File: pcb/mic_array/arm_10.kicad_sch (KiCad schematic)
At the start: 16 parts, among them U81 IM72D128V01XTMA1, U82 IM72D128V01XTMA1, U83 IM72D128V01XTMA1, U84 IM72D128V01XTMA1, U85 IM72D128V01XTMA1, U86 IM72D128V01XTMA1, U87 IM72D128V01XTMA1, U88 IM72D128V01XTMA1

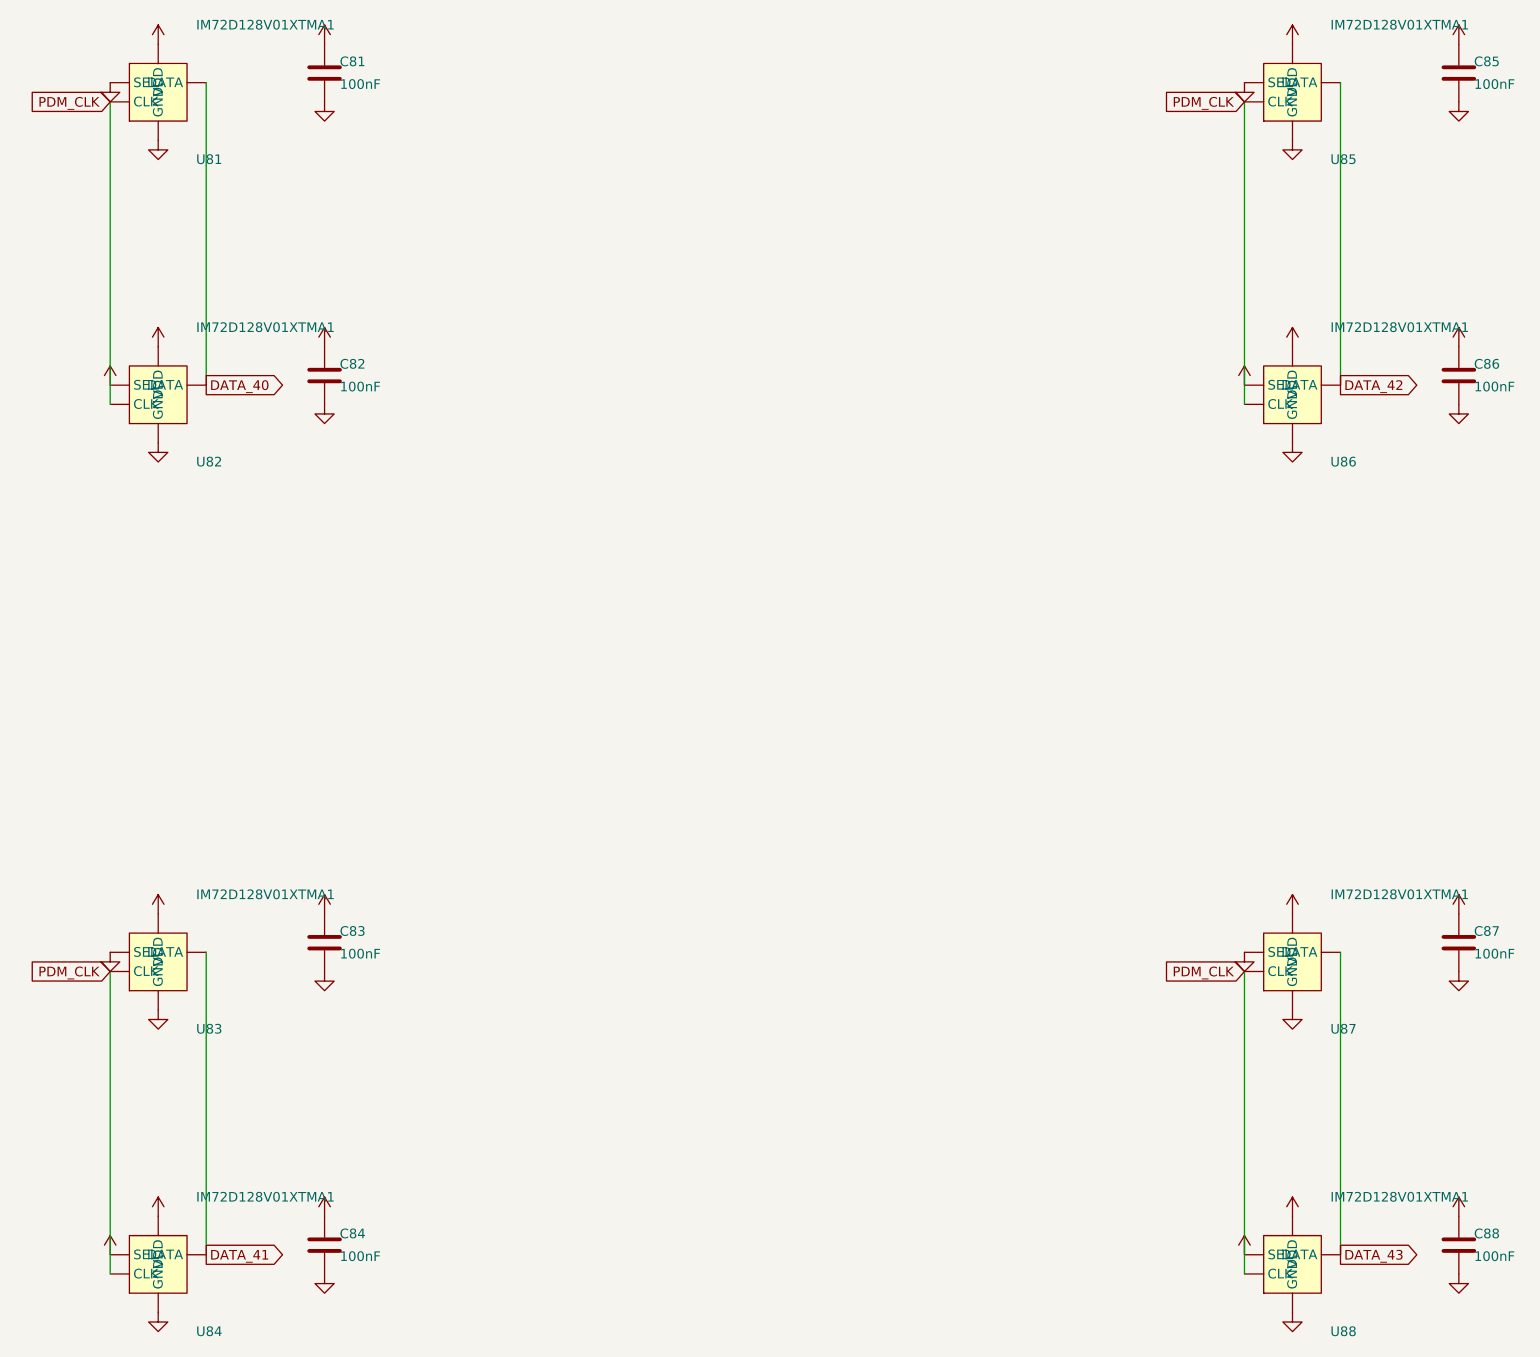
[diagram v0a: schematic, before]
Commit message: Updated.
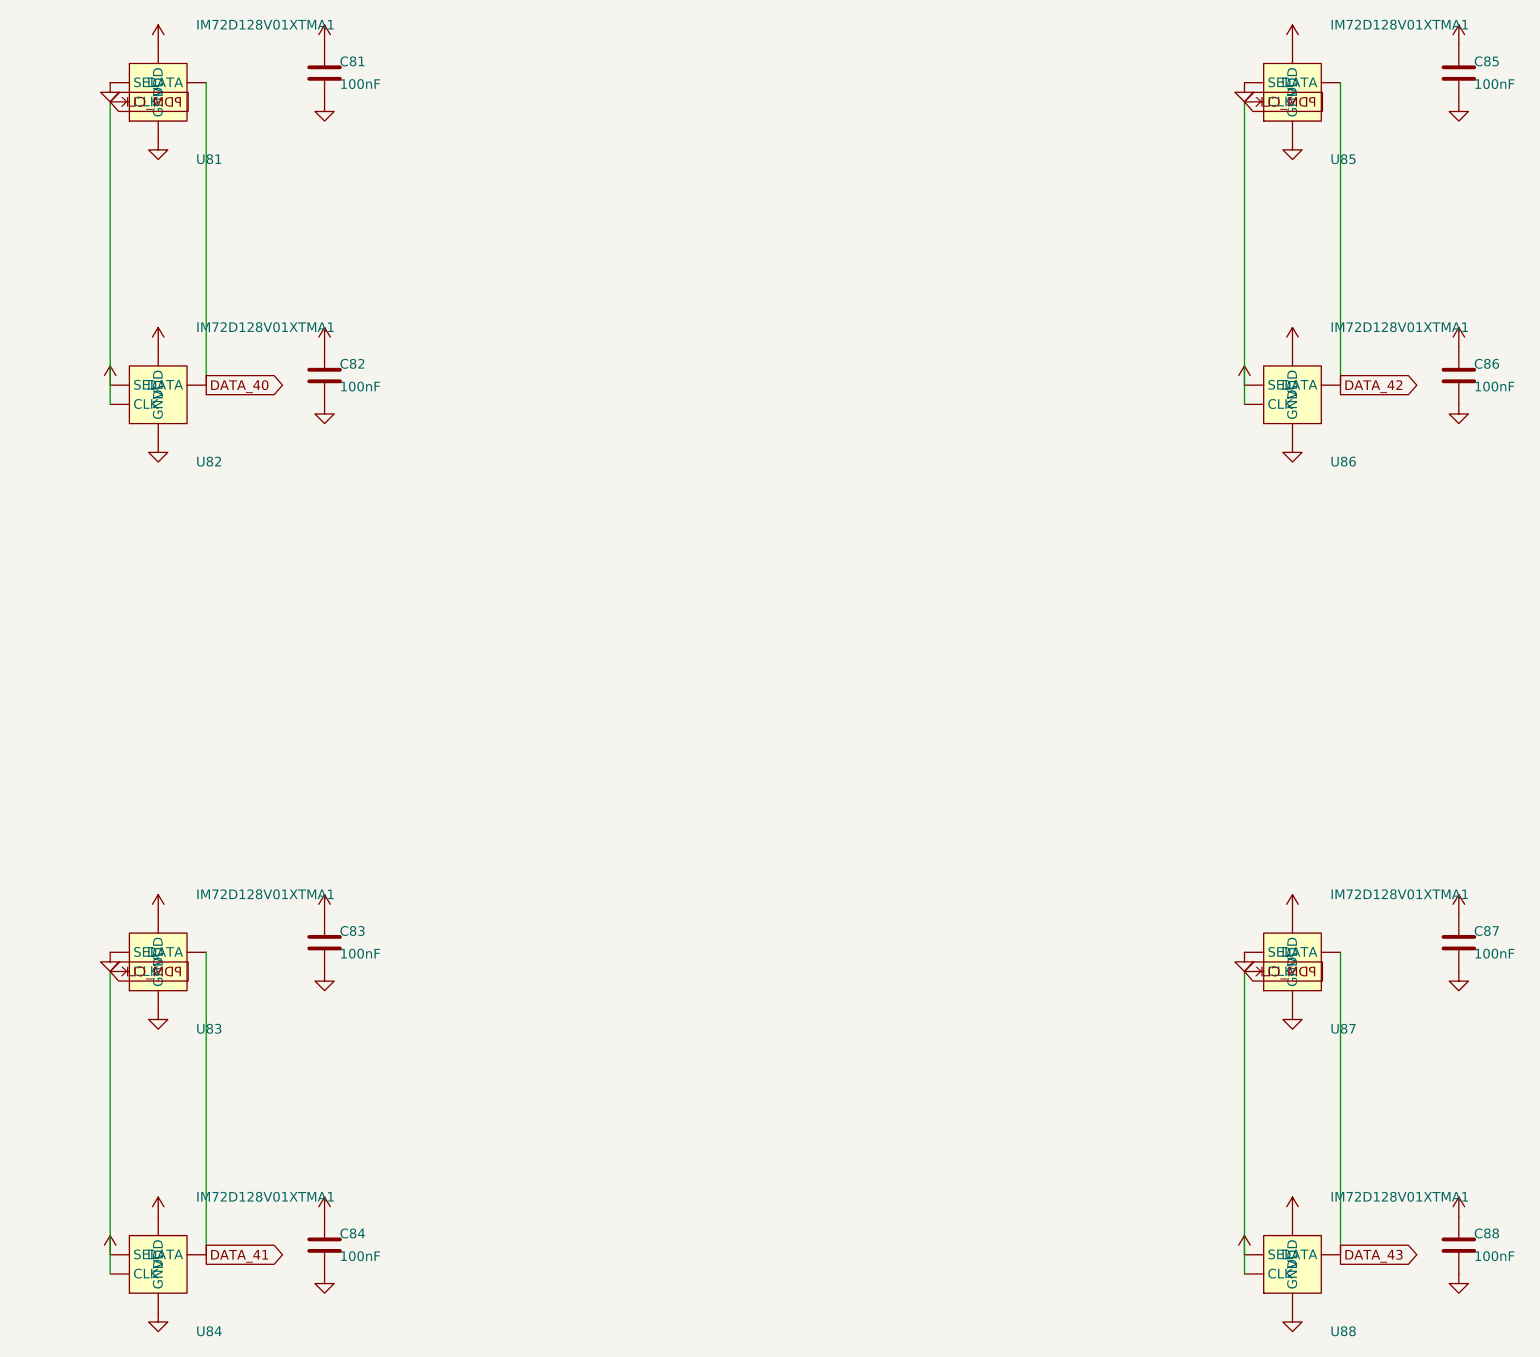
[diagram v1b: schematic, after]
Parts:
- C81, C82, C83, C84, C85, C86, C87, C88: footprint Capacitor_SMD:C_0402_1005Metric -> (none)
- U81, U82, U83, U84, U85, U86, U87, U88: footprint Sensor_Audio:Infineon_PG-LLGA-5-2 -> (none)
